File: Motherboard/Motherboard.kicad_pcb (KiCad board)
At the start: 8 copper layers, 508 x 330.2 mm, 192 parts, among them J1 Jack-DC_18v, J2 65SIB_Connector, J3 DB9_Header, J4 GPIO_Connector, J5 Expansion_Connector, J6 Expansion_Connector, J7 Expansion_Connector, J8 Expansion_Connector, J9 Expansion_Connector, P1 POWER TERMINAL, Q1 2N3055, Q2 TIC106, SW1 SW_DPDT, SW2 FUSE RESET, SW3 PROCESSOR RESET, U1 LM7812_TO220, U13 LM386, U14 LM7912_TO220, U4 LM7805_TO220, X1 ACO-8MHz

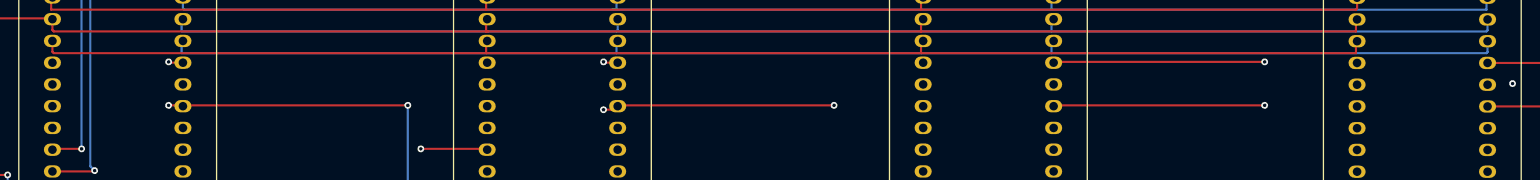
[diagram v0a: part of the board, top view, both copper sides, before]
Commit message: 156 unrouted traces...
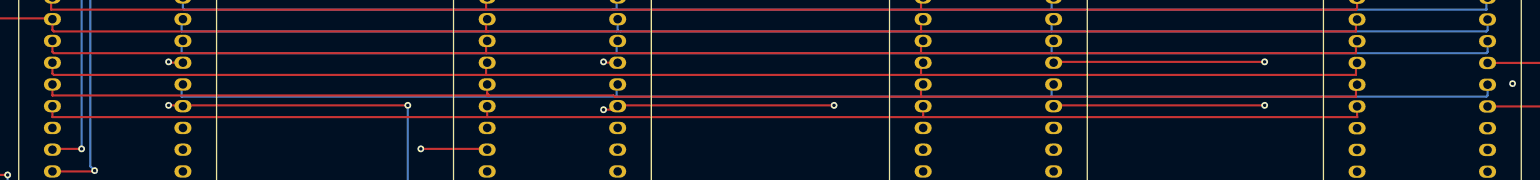
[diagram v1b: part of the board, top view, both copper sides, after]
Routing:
- net A10: track 649.1 -> 807.5 mm
- net A2: track 791.0 -> 949.1 mm
- net A3: track 917.8 -> 1075.9 mm
- net A1: track 792.2 -> 949.7 mm
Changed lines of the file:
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@@
     (thickness 4)
     (drawings 14)
-    (tracks 4716)
+    (tracks 4763)
     (zones 0)
     (modules 192)
@@
   (segment (start 320.7004 334.6704) (end 320.7004 335.788) (width 0.25) (layer SIGV.Cu) (net 57))
   (segment (start 371.348 335.788) (end 320.548 335.788) (width 0.25) (layer SIGV.Cu) (net 57))
+  (segment (start 473.075 267.335) (end 473.075 268.605) (width 0.25) (layer SIGV.Cu) (net 57))
+  (segment (start 473.075 268.605) (end 472.948 268.732) (width 0.25) (layer SIGV.Cu) (net 57))
+  (segment (start 472.948 268.732) (end 422.148 268.732) (width 0.25) (layer SIGV.Cu) (net 57))
+  (segment (start 422.148 267.552) (end 422.395 267.305) (width 0.25) (layer SIGV.Cu) (net 57))
+  (segment (start 422.148 268.732) (end 422.148 267.552) (width 0.25) (layer SIGV.Cu) (net 57))
+  (segment (start 371.348 268.732) (end 422.148 268.732) (width 0.25) (layer SIGV.Cu) (net 57))
+  (segment (start 371.348 267.432) (end 371.348 268.732) (width 0.25) (layer SIGV.Cu) (net 57))
+  (segment (start 371.475 267.305) (end 371.348 267.432) (width 0.25) (layer SIGV.Cu) (net 57))
+  (segment (start 371.348 268.732) (end 320.548 268.732) (width 0.25) (layer SIGV.Cu) (net 57))
+  (segment (start 320.548 267.457) (end 320.7 267.305) (width 0.25) (layer SIGV.Cu) (net 57))
+  (segment (start 320.548 268.732) (end 320.548 267.457) (width 0.25) (layer SIGV.Cu) (net 57))
   (via (at 215.9 342.9) (size 0.8) (drill 0.4) (layers SIGH.Cu SIGV.Cu) (net 58))
   (segment (start 222.9104 342.9) (end 215.9 342.9) (width 0.25) (layer SIGH.Cu) (net 58) (status 10))
@@
   (segment (start 508.508 333.248) (end 508.508 332.2828) (width 0.25) (layer SIGH.Cu) (net 70))
   (segment (start 457.708 333.248) (end 508.508 333.248) (width 0.25) (layer SIGH.Cu) (net 70))
+  (segment (start 356.108 266.192) (end 356.108 264.892) (width 0.25) (layer SIGH.Cu) (net 70))
+  (segment (start 305.612 266.192) (end 356.108 266.192) (width 0.25) (layer SIGH.Cu) (net 70))
+  (segment (start 356.108 264.892) (end 356.235 264.765) (width 0.25) (layer SIGH.Cu) (net 70))
+  (segment (start 305.46 266.04) (end 305.612 266.192) (width 0.25) (layer SIGH.Cu) (net 70))
+  (segment (start 305.46 264.765) (end 305.46 266.04) (width 0.25) (layer SIGH.Cu) (net 70))
+  (segment (start 406.908 265.012) (end 407.155 264.765) (width 0.25) (layer SIGH.Cu) (net 70))
+  (segment (start 406.908 266.192) (end 406.908 265.012) (width 0.25) (layer SIGH.Cu) (net 70))
+  (segment (start 356.108 266.192) (end 406.908 266.192) (width 0.25) (layer SIGH.Cu) (net 70))
+  (segment (start 406.908 266.192) (end 457.708 266.192) (width 0.25) (layer SIGH.Cu) (net 70))
+  (segment (start 457.708 264.922) (end 457.835 264.795) (width 0.25) (layer SIGH.Cu) (net 70))
+  (segment (start 457.708 266.192) (end 457.708 264.922) (width 0.25) (layer SIGH.Cu) (net 70))
   (segment (start 522.6304 57.8104) (end 522.6304 59.0296) (width 0.25) (layer SIGV.Cu) (net 71) (status 10))
   (segment (start 522.6304 59.0296) (end 522.605 59.055) (width 0.25) (layer SIGV.Cu) (net 71))
@@
   (segment (start 508.508 334.8228) (end 508.6604 334.6704) (width 0.25) (layer SIGH.Cu) (net 72))
   (segment (start 508.508 335.788) (end 508.508 334.8228) (width 0.25) (layer SIGH.Cu) (net 72))
+  (segment (start 356.235 268.321) (end 356.235 267.305) (width 0.25) (layer SIGH.Cu) (net 72))
+  (segment (start 356.235 268.351) (end 356.235 268.321) (width 0.25) (layer SIGH.Cu) (net 72))
+  (segment (start 356.474 268.59) (end 356.235 268.351) (width 0.25) (layer SIGH.Cu) (net 72))
+  (segment (start 305.46 268.58) (end 305.47 268.59) (width 0.25) (layer SIGH.Cu) (net 72))
+  (segment (start 305.46 267.305) (end 305.46 268.58) (width 0.25) (layer SIGH.Cu) (net 72))
+  (segment (start 305.47 268.59) (end 356.25 268.59) (width 0.25) (layer SIGH.Cu) (net 72))
+  (segment (start 356.25 268.59) (end 356.474 268.59) (width 0.25) (layer SIGH.Cu) (net 72))
+  (segment (start 406.908 267.552) (end 407.155 267.305) (width 0.25) (layer SIGH.Cu) (net 72))
+  (segment (start 406.908 268.732) (end 406.908 267.552) (width 0.25) (layer SIGH.Cu) (net 72))
+  (segment (start 371.124 268.732) (end 406.908 268.732) (width 0.25) (layer SIGH.Cu) (net 72))
+  (segment (start 370.982 268.59) (end 371.124 268.732) (width 0.25) (layer SIGH.Cu) (net 72))
+  (segment (start 356.25 268.59) (end 370.982 268.59) (width 0.25) (layer SIGH.Cu) (net 72))
+  (segment (start 406.908 268.732) (end 457.708 268.732) (width 0.25) (layer SIGH.Cu) (net 72))
+  (segment (start 457.708 267.462) (end 457.835 267.335) (width 0.25) (layer SIGH.Cu) (net 72))
+  (segment (start 457.708 268.732) (end 457.708 267.462) (width 0.25) (layer SIGH.Cu) (net 72))
   (segment (start 497.205 56.515) (end 497.205 55.2958) (width 0.25) (layer SIGV.Cu) (net 73) (status 20))
   (segment (start 522.605 56.515) (end 497.205 56.515) (width 0.25) (layer SIGV.Cu) (net 73))
@@
   (segment (start 508.43541 338.25541) (end 508.43541 337.43539) (width 0.25) (layer SIGH.Cu) (net 74))
   (segment (start 457.63541 338.25541) (end 508.43541 338.25541) (width 0.25) (layer SIGH.Cu) (net 74))
+  (segment (start 305.46 269.845) (end 305.46 271.12) (width 0.25) (layer SIGH.Cu) (net 74))
+  (segment (start 305.46 271.12) (end 356.26 271.12) (width 0.25) (layer SIGH.Cu) (net 74))
+  (segment (start 356.235 271.095) (end 356.235 269.845) (width 0.25) (layer SIGH.Cu) (net 74))
+  (segment (start 356.26 271.12) (end 356.235 271.095) (width 0.25) (layer SIGH.Cu) (net 74))
+  (segment (start 356.26 271.12) (end 407.264 271.12) (width 0.25) (layer SIGH.Cu) (net 74))
+  (segment (start 407.155 271.011) (end 407.155 269.845) (width 0.25) (layer SIGH.Cu) (net 74))
+  (segment (start 407.264 271.12) (end 407.155 271.011) (width 0.25) (layer SIGH.Cu) (net 74))
+  (segment (start 407.264 271.12) (end 457.86 271.12) (width 0.25) (layer SIGH.Cu) (net 74))
+  (segment (start 457.835 271.095) (end 457.835 269.875) (width 0.25) (layer SIGH.Cu) (net 74))
+  (segment (start 457.86 271.12) (end 457.835 271.095) (width 0.25) (layer SIGH.Cu) (net 74))
   (segment (start 497.205 52.7558) (end 497.2304 52.7304) (width 0.25) (layer SIGV.Cu) (net 75) (status 30))
   (segment (start 497.205 53.975) (end 497.205 52.7558) (width 0.25) (layer SIGV.Cu) (net 75) (status 20))
